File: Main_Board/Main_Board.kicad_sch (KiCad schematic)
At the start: 0 parts

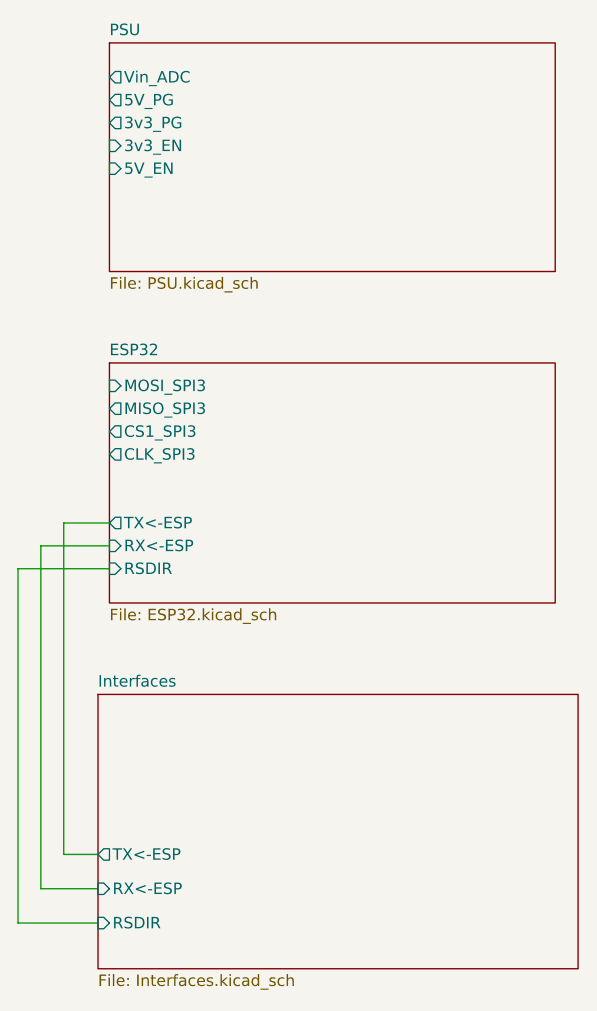
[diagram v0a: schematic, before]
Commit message: Aesthetics/cleanup
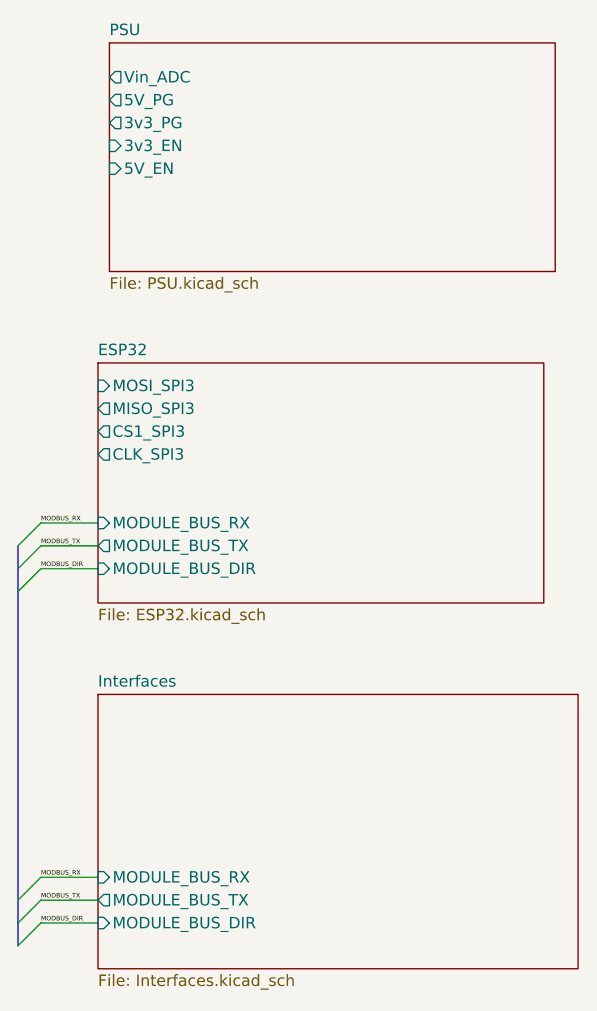
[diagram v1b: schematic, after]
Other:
- sheet ESP32 ports: added MODULE_BUS_DIR, MODULE_BUS_RX, MODULE_BUS_TX; removed RSDIR, RX<-ESP, TX<-ESP
- sheet Interfaces ports: added MODULE_BUS_DIR, MODULE_BUS_RX, MODULE_BUS_TX; removed RSDIR, RX<-ESP, TX<-ESP
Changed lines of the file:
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@@
 	(generator_version "10.0")
 	(paper "A4")
-	(wire
-		(pts
-			(xy 190.5 93.98) (xy 182.88 93.98)
-		)
-		(stroke
-			(width 0)
-			(type default)
-		)
-	)
-	(wire
-		(pts
-			(xy 180.34 96.52) (xy 180.34 135.89)
-		)
-		(stroke
-			(width 0)
-			(type default)
-		)
-	)
-	(wire
-		(pts
-			(xy 185.42 91.44) (xy 185.42 128.27)
-		)
-		(stroke
-			(width 0)
-			(type default)
-		)
-	)
-	(wire
-		(pts
-			(xy 190.5 91.44) (xy 185.42 91.44)
-		)
-		(stroke
-			(width 0)
-			(type default)
-		)
-	)
-	(wire
-		(pts
-			(xy 190.5 96.52) (xy 180.34 96.52)
-		)
-		(stroke
-			(width 0)
-			(type default)
-		)
-	)
-	(wire
-		(pts
-			(xy 182.88 93.98) (xy 182.88 132.08)
-		)
-		(stroke
-			(width 0)
-			(type default)
-		)
-	)
-	(wire
-		(pts
-			(xy 182.88 132.08) (xy 189.23 132.08)
-		)
-		(stroke
-			(width 0)
-			(type default)
-		)
-	)
-	(wire
-		(pts
-			(xy 180.34 135.89) (xy 189.23 135.89)
-		)
-		(stroke
-			(width 0)
-			(type default)
-		)
-	)
-	(wire
-		(pts
-			(xy 185.42 128.27) (xy 189.23 128.27)
-		)
-		(stroke
-			(width 0)
-			(type default)
+	(bus_entry
+		(at 182.88 91.44)
+		(size -2.54 2.54)
+		(stroke
+			(width 0)
+			(type default)
+		)
+	)
+	(bus_entry
+		(at 182.88 130.81)
+		(size -2.54 2.54)
+		(stroke
+			(width 0)
+			(type default)
+		)
+	)
+	(bus_entry
+		(at 182.88 96.52)
+		(size -2.54 2.54)
+		(stroke
+			(width 0)
+			(type default)
+		)
+	)
+	(bus_entry
+		(at 182.88 93.98)
+		(size -2.54 2.54)
+		(stroke
+			(width 0)
+			(type default)
+		)
+	)
+	(bus_entry
+		(at 182.88 133.35)
+		(size -2.54 2.54)
+		(stroke
+			(width 0)
+			(type default)
+		)
+	)
+	(bus_entry
+		(at 182.88 135.89)
+		(size -2.54 2.54)
+		(stroke
+			(width 0)
+			(type default)
+		)
+	)
+	(wire
+		(pts
+			(xy 182.88 91.44) (xy 189.23 91.44)
+		)
+		(stroke
+			(width 0)
+			(type default)
+		)
+	)
+	(wire
+		(pts
+			(xy 182.88 133.35) (xy 189.23 133.35)
+		)
+		(stroke
+			(width 0)
+			(type default)
+		)
+	)
+	(wire
+		(pts
+			(xy 182.88 130.81) (xy 189.23 130.81)
+		)
+		(stroke
+			(width 0)
+			(type default)
+		)
+	)
+	(bus
+		(pts
+			(xy 180.34 93.98) (xy 180.34 99.06)
+		)
+		(stroke
+			(width 0)
+			(type default)
+		)
+	)
+	(wire
+		(pts
+			(xy 182.88 135.89) (xy 189.23 135.89)
+		)
+		(stroke
+			(width 0)
+			(type default)
+		)
+	)
+	(wire
+		(pts
+			(xy 182.88 96.52) (xy 189.23 96.52)
+		)
+		(stroke
+			(width 0)
+			(type default)
+		)
+	)
+	(wire
+		(pts
+			(xy 182.88 93.98) (xy 189.23 93.98)
+		)
+		(stroke
+			(width 0)
+			(type default)
+		)
+	)
+	(bus
+		(pts
+			(xy 180.34 135.89) (xy 180.34 138.43)
+		)
+		(stroke
+			(width 0)
+			(type default)
+		)
+	)
+	(bus
+		(pts
+			(xy 180.34 99.06) (xy 180.34 135.89)
+		)
+		(stroke
+			(width 0)
+			(type default)
+		)
+	)
+	(label "MODBUS_DIR"
+		(at 182.88 96.52 0)
+		(effects
+			(font
+				(size 0.508 0.508)
+			)
+			(justify left bottom)
+		)
+	)
+	(label "MODBUS_RX"
+		(at 182.88 91.44 0)
+		(effects
+			(font
+				(size 0.508 0.508)
+			)
+			(justify left bottom)
+		)
+	)
+	(label "MODBUS_DIR"
+		(at 182.88 135.89 0)
+		(effects
+			(font
+				(size 0.508 0.508)
+			)
+			(justify left bottom)
+		)
+	)
+	(label "MODBUS_TX"
+		(at 182.88 133.35 0)
+		(effects
+			(font
+				(size 0.508 0.508)
+			)
+			(justify left bottom)
+		)
+	)
+	(label "MODBUS_TX"
+		(at 182.88 93.98 0)
+		(effects
+			(font
+				(size 0.508 0.508)
+			)
+			(justify left bottom)
+		)
+	)
+	(label "MODBUS_RX"
+		(at 182.88 130.81 0)
+		(effects
+			(font
+				(size 0.508 0.508)
+			)
+			(justify left bottom)
 		)
 	)
@@
 	)
 	(sheet
-		(at 190.5 73.66)
+		(at 189.23 73.66)
 		(size 49.53 26.67)
 		(exclude_from_sim no)
@@
 		)
 		(property "Sheetname" "ESP32"
-			(at 190.5 72.9484 0)
+			(at 189.23 72.9484 0)
 			(show_name no)
 			(do_not_autoplace no)
@@
 		)
 		(property "Sheetfile" "ESP32.kicad_sch"
-			(at 190.5 100.9146 0)
+			(at 189.23 100.9146 0)
 			(show_name no)
 			(do_not_autoplace no)
@@
 			)
 		)
-		(pin "TX<-ESP" output
-			(at 190.5 91.44 180)
-			(effects
-				(font
-					(size 1.27 1.27)
-				)
-				(justify left)
-			)
-		)
-		(pin "RX<-ESP" input
-			(at 190.5 93.98 180)
-			(effects
-				(font
-					(size 1.27 1.27)
-				)
-				(justify left)
-			)
-		)
 		(pin "MOSI_SPI3" input
-			(at 190.5 76.2 180)
+			(at 189.23 76.2 180)
 			(effects
 				(font
@@
 		)
 		(pin "MISO_SPI3" output
-			(at 190.5 78.74 180)
+			(at 189.23 78.74 180)
 			(effects
 				(font
@@
 		)
 		(pin "CS1_SPI3" output
-			(at 190.5 81.28 180)
+			(at 189.23 81.28 180)
 			(effects
 				(font
@@
 		)
 		(pin "CLK_SPI3" output
-			(at 190.5 83.82 180)
-			(effects
-				(font
-					(size 1.27 1.27)
-				)
-				(justify left)
-			)
-		)
-		(pin "RSDIR" input
-			(at 190.5 96.52 180)
+			(at 189.23 83.82 180)
+			(effects
+				(font
+					(size 1.27 1.27)
+				)
+				(justify left)
+			)
+		)
+		(pin "MODULE_BUS_RX" input
+			(at 189.23 91.44 180)
+			(effects
+				(font
+					(size 1.27 1.27)
+				)
+				(justify left)
+			)
+		)
+		(pin "MODULE_BUS_DIR" input
+			(at 189.23 96.52 180)
+			(effects
+				(font
+					(size 1.27 1.27)
+				)
+				(justify left)
+			)
+		)
+		(pin "MODULE_BUS_TX" output
+			(at 189.23 93.98 180)
 			(effects
 				(font
@@
 			)
 		)
-		(pin "RSDIR" input
+		(pin "MODULE_BUS_RX" input
+			(at 189.23 130.81 180)
+			(effects
+				(font
+					(size 1.27 1.27)
+				)
+				(justify left)
+			)
+		)
+		(pin "MODULE_BUS_TX" output
+			(at 189.23 133.35 180)
+			(effects
+				(font
+					(size 1.27 1.27)
+				)
+				(justify left)
+			)
+		)
+		(pin "MODULE_BUS_DIR" input
 			(at 189.23 135.89 180)
 			(effects
 				(font
-					(size 1.27 1.27)
-				)
-				(justify left)
-			)
-		)
-		(pin "RX<-ESP" input
-			(at 189.23 132.08 180)
-			(effects
-				(font
-					(size 1.27 1.27)
-				)
-				(justify left)
-			)
-		)
-		(pin "TX<-ESP" output
-			(at 189.23 128.27 180)
-			(effects
-				(font
